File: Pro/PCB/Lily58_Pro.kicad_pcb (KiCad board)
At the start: 2 copper layers, 142.5 x 106.3 mm, 87 parts, among them J1 LED, J2 4PIN, J3 OLED, P1 i2c_pin, P2 i2c_pin, SW1 SW_PUSH, SW10 SW_PUSH, SW11 SW_PUSH, SW12 SW_PUSH, SW13 SW_PUSH, SW14 SW_PUSH, SW15 SW_PUSH, SW16 SW_PUSH, SW17 SW_PUSH, SW18 SW_PUSH, SW19 SW_PUSH, SW2 SW_PUSH, SW20 SW_PUSH, SW21 SW_PUSH, SW22 SW_PUSH, SW23 SW_PUSH, SW24 SW_PUSH, SW25 SW_PUSH, SW26 SW_PUSH, SW27 SW_PUSH, SW28 SW_PUSH, SW29 SW_PUSH, SW3 SW_PUSH, SW4 SW_PUSH, SW5 SW_PUSH, SW6 SW_PUSH, SW7 SW_PUSH, SW8 SW_PUSH, SW9 SW_PUSH, U1 ProMicro

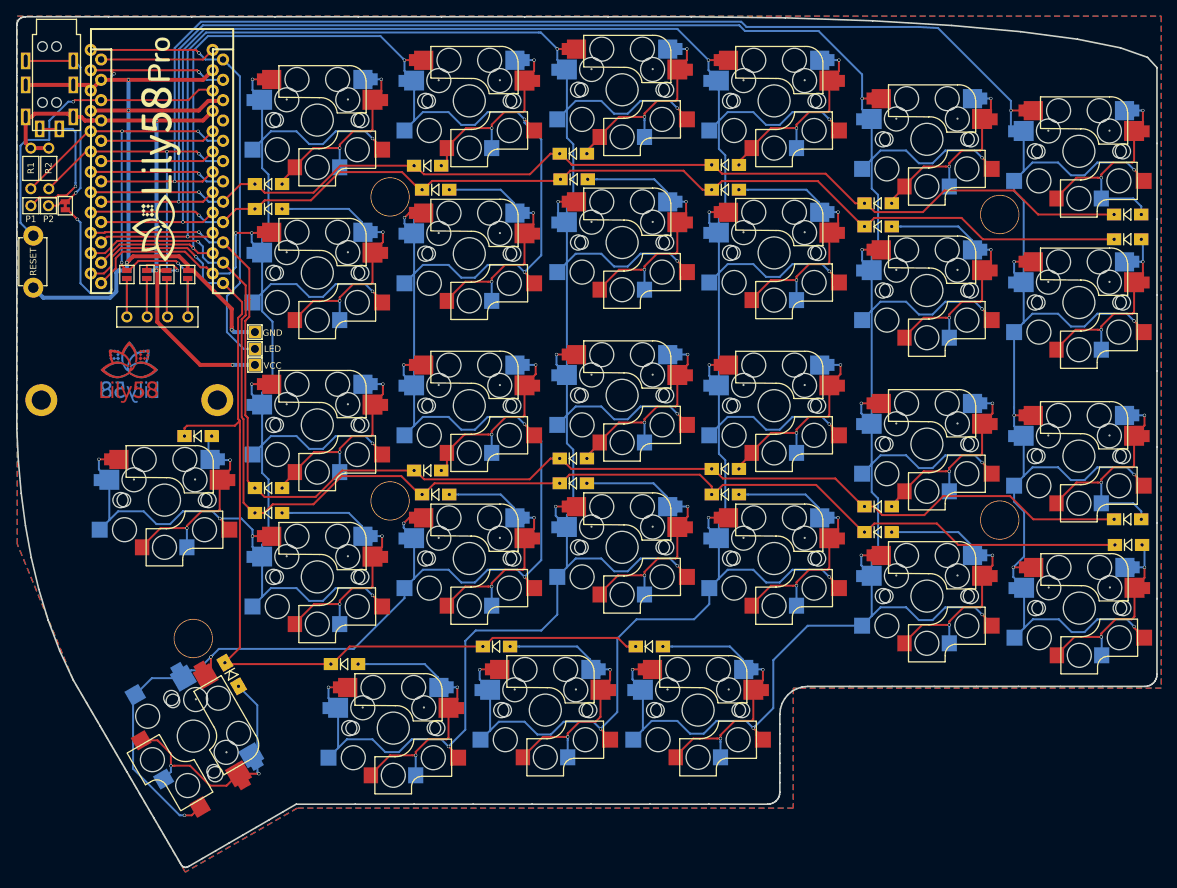
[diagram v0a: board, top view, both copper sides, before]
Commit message: Lily58 Choc full backlight edition
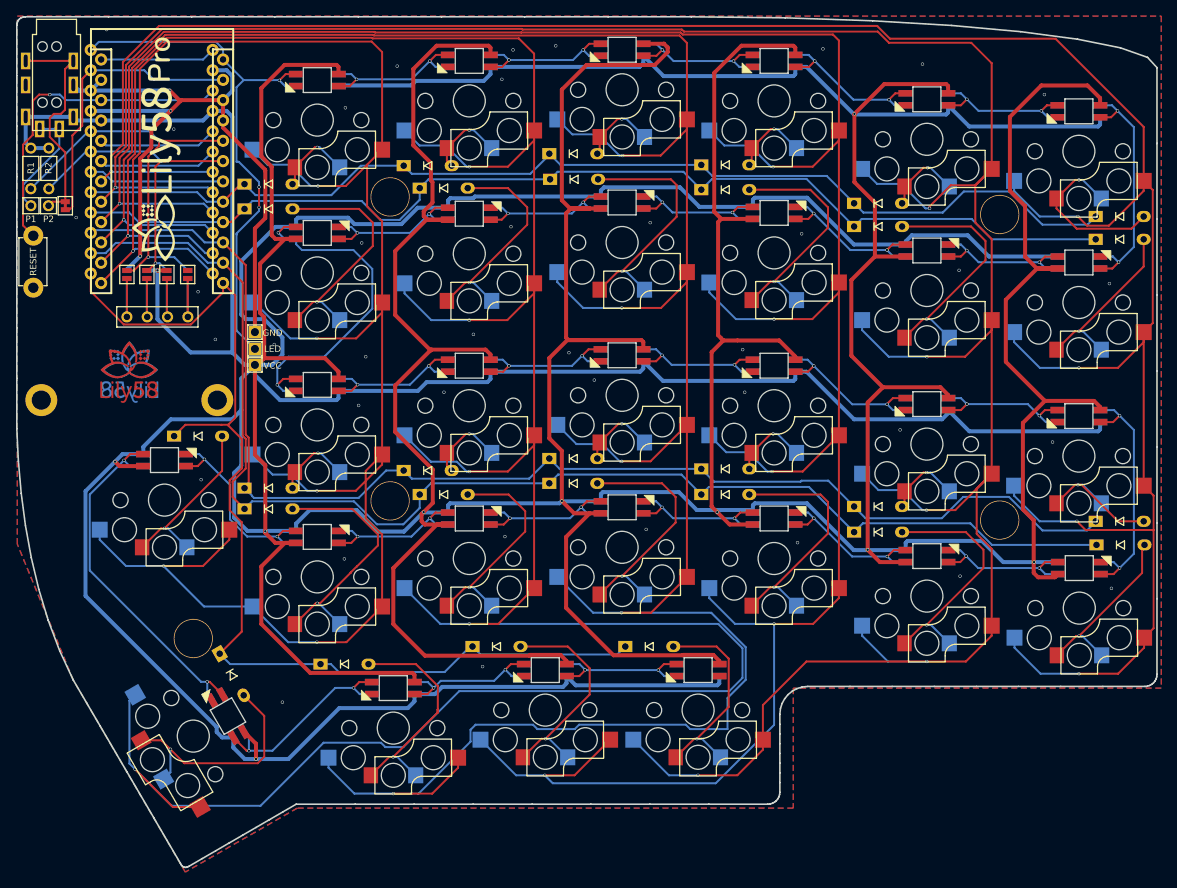
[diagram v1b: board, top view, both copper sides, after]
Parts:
- added LED1: SK6812MINI-E, Lily58_Pro-footprint:SK6812MINI-E_both, F.Cu at (120.5, 45.0)
- added LED10: SK6812MINI-E, Lily58_Pro-footprint:SK6812MINI-E_both, F.Cu at (177.6, 61.6)
- added LED11: SK6812MINI-E, Lily58_Pro-footprint:SK6812MINI-E_both, F.Cu at (196.7, 66.3)
- added LED12: SK6812MINI-E, Lily58_Pro-footprint:SK6812MINI-E_both, F.Cu at (215.7, 67.8)
- added LED13: SK6812MINI-E, Lily58_Pro-footprint:SK6812MINI-E_both, F.Cu at (120.5, 83.1)
- added LED14: SK6812MINI-E, Lily58_Pro-footprint:SK6812MINI-E_both, F.Cu at (139.5, 80.7)
- added LED15: SK6812MINI-E, Lily58_Pro-footprint:SK6812MINI-E_both, F.Cu at (158.6, 79.4)
- added LED16: SK6812MINI-E, Lily58_Pro-footprint:SK6812MINI-E_both, F.Cu at (177.6, 80.7)
- added LED17: SK6812MINI-E, Lily58_Pro-footprint:SK6812MINI-E_both, F.Cu at (196.7, 85.5)
- added LED18: SK6812MINI-E, Lily58_Pro-footprint:SK6812MINI-E_both, B.Cu at (215.7, 87.0)
- added LED19: SK6812MINI-E, Lily58_Pro-footprint:SK6812MINI-E_both, F.Cu at (120.5, 102.1)
- added LED2: SK6812MINI-E, Lily58_Pro-footprint:SK6812MINI-E_both, F.Cu at (139.5, 42.6)
- added LED20: SK6812MINI-E, Lily58_Pro-footprint:SK6812MINI-E_both, F.Cu at (139.5, 99.8)
- added LED21: SK6812MINI-E, Lily58_Pro-footprint:SK6812MINI-E_both, F.Cu at (158.6, 98.4)
- added LED22: SK6812MINI-E, Lily58_Pro-footprint:SK6812MINI-E_both, F.Cu at (177.6, 99.8)
- added LED23: SK6812MINI-E, Lily58_Pro-footprint:SK6812MINI-E_both, F.Cu at (196.7, 104.5)
- added LED24: SK6812MINI-E, Lily58_Pro-footprint:SK6812MINI-E_both, F.Cu at (215.8, 106.0)
- added LED25: SK6812MINI-E, Lily58_Pro-footprint:SK6812MINI-E_both, F.Cu at (101.4, 92.5)
- added LED26: SK6812MINI-E, Lily58_Pro-footprint:SK6812MINI-E_both, F.Cu at (109.3, 124.5)
- added LED27: SK6812MINI-E, Lily58_Pro-footprint:SK6812MINI-E_both, F.Cu at (130.0, 121.0)
- added LED28: SK6812MINI-E, Lily58_Pro-footprint:SK6812MINI-E_both, F.Cu at (149.0, 118.8)
- added LED29: SK6812MINI-E, Lily58_Pro-footprint:SK6812MINI-E_both, F.Cu at (168.1, 118.8)
- added LED3: SK6812MINI-E, Lily58_Pro-footprint:SK6812MINI-E_both, F.Cu at (158.6, 41.2)
- added LED4: SK6812MINI-E, Lily58_Pro-footprint:SK6812MINI-E_both, F.Cu at (177.6, 42.6)
- added LED5: SK6812MINI-E, Lily58_Pro-footprint:SK6812MINI-E_both, F.Cu at (196.7, 47.4)
- added LED6: SK6812MINI-E, Lily58_Pro-footprint:SK6812MINI-E_both, F.Cu at (215.7, 48.9)
- added LED7: SK6812MINI-E, Lily58_Pro-footprint:SK6812MINI-E_both, F.Cu at (120.5, 64.1)
- added LED8: SK6812MINI-E, Lily58_Pro-footprint:SK6812MINI-E_both, F.Cu at (139.5, 61.7)
- added LED9: SK6812MINI-E, Lily58_Pro-footprint:SK6812MINI-E_both, F.Cu at (158.6, 60.3)
- D1, D10, D11, D12, D13, D14, D15, D16, D17, D18, D19, D2, D20, D21, D22, D23, D24, D25, D26, D27, D28, D29, D3, D4, D5, D6, D7, D8, D9: footprint Lily58-footprint:Diode_SOD123 -> kbd:D3_TH
- JP1, JP2, JP3, JP4, JP5, JP6, JP7, JP8: value (none) -> Jumper_NO_Small
- SW1, SW10, SW11, SW12, SW13, SW14, SW15, SW16, SW17, SW18, SW19, SW2, SW20, SW21, SW22, SW23, SW24, SW25, SW26, SW27, SW28, SW29, SW3, SW4, SW5, SW6, SW7, SW8, SW9: footprint Lily58-footprint:CherryMX_KailhLowProfile_Hotswap_edge -> Lily58_Pro-footprint:Choc_Hotswap_both
- moved D18 1.03 mm to (220.8, 100.2)
- moved D6 1.03 mm to (220.8, 62.0)
- moved D8 1.02 mm to (136.3, 58.5)
- moved D12 1.00 mm to (220.8, 64.9)
- moved D20 1.00 mm to (136.3, 96.8)
- moved D24 1.00 mm to (220.9, 103.1)
- moved D19 0.50 mm to (114.4, 98.6)
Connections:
- U1 pad 19: Net-(U1-Pad19) -> unconnected-(U1-Pad19)
- U1 pad 20: Net-(U1-Pad20) -> unconnected-(U1-Pad20)
- U1 pad 24: Net-(U1-Pad24) -> unconnected-(U1-Pad24)
- U1 pad 7: Net-(U1-Pad7) -> unconnected-(U1-Pad7)
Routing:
- net VCC: track 72.9 -> 1389.3 mm, vias 3 -> 10
- net col4: track 319.5 -> 383.3 mm, vias 11 -> 6
- net Net-(LED25-Pad2): track 0.00 -> 46.7 mm, vias 0 -> 2
- net Net-(LED13-Pad4): track 0.00 -> 43.9 mm, vias 0 -> 2
- net col3: track 319.9 -> 352.1 mm, vias 11 -> 6
- net Net-(LED18-Pad2): track 0.00 -> 31.4 mm, vias 0 -> 2
- net Net-(LED12-Pad4): track 0.00 -> 30.8 mm, vias 0 -> 2
- net Net-(LED26-Pad2): track 0.00 -> 26.9 mm, vias 0 -> 2
- net Net-(LED19-Pad2): track 0.00 -> 26.3 mm, vias 0 -> 2
- net DATA: track 59.7 -> 36.1 mm, vias 3 -> 0
- net Net-(LED13-Pad2): track 0.00 -> 22.3 mm, vias 0 -> 2
- net col5: track 235.9 -> 258.1 mm, vias 11 -> 6
- net Net-(LED27-Pad2): track 0.00 -> 22.2 mm, vias 0 -> 2
- net Net-(LED16-Pad2): track 0.00 -> 21.7 mm, vias 0 -> 2
- net Net-(LED22-Pad4): track 0.00 -> 21.6 mm, vias 0 -> 2
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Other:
- net class Default removed
- net class GND removed
- net class VCC removed
